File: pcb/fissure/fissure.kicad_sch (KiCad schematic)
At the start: 64 parts, among them J1 Conn_01x04_Female, J2 USB_C_Receptacle_USB2.0, J3 Conn_01x06, J4 Conn_01x06, J5 OLED, J6 Conn_01x06, J7 Conn_01x06, K1 KEY, K10 KEY, K11 KEY, K12 KEY, K13 KEY, K14 KEY, K15 KEY, K16 KEY, K17 KEY, K18 KEY, K19 KEY, K2 KEY, K20 KEY, K3 KEY, K4 KEY, K5 KEY, K6 KEY, K7 KEY, K8 KEY, K9 KEY, Q1 AO3401A, Q2 AO3401A, SW1 SW_Push, SW2 SW_Push, SW3 SW_SPDT, SW4 SW_SPDT, U1 Holyiot_18010, U2 MT25QL128ABA1ESE, U3 LTC4054ES5-4.2, U4 MCP1700-3302E_SOT23

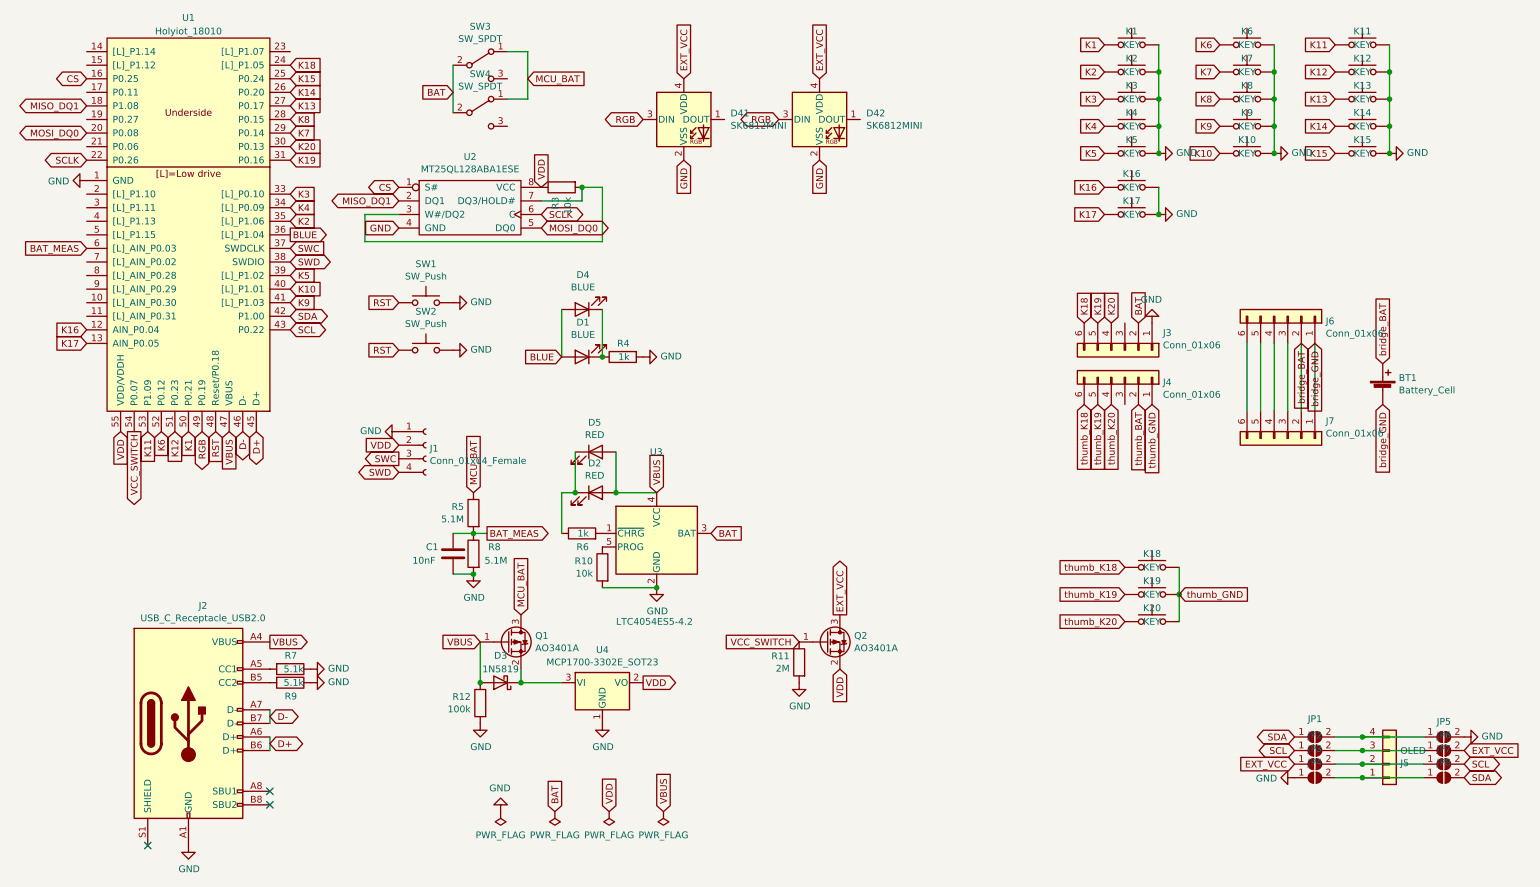
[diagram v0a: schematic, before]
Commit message: Backup
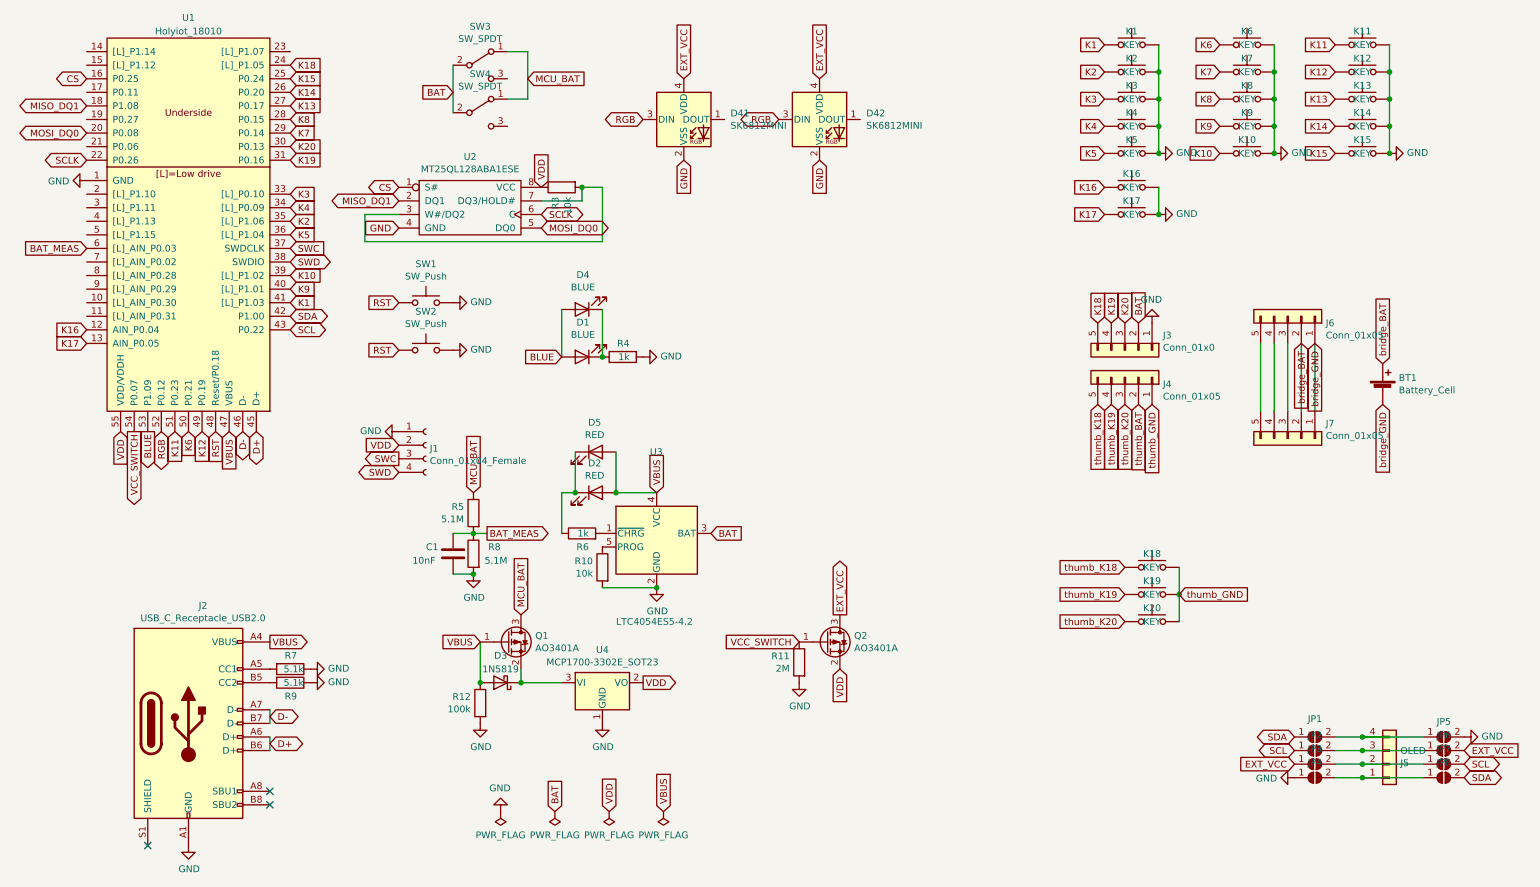
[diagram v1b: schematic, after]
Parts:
- removed J3, J4: Conn_01x06, fissure:bridge-conn, symbol Connector_Generic:Conn_01x06
- removed J6, J7: Conn_01x06, fissure:bridge, symbol Connector_Generic:Conn_01x06
- added J3: Conn_01x0, fissure:bridge-conn, symbol Connector_Generic:Conn_01x05
- added J4: Conn_01x05, fissure:bridge-conn, symbol Connector_Generic:Conn_01x05
- added J6, J7: Conn_01x05, fissure:bridge, symbol Connector_Generic:Conn_01x05
- D1, D2, D4, D5: footprint LED_SMD:LED_1206_3216Metric -> LED_SMD:LED_0805_2012Metric
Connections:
- net BAT: now also J3.2 (Pin_2)
- net BLUE: now also U1.53 (P1.09); no longer U1.36 ([L]_P1.04)
- net GND: now also J3.1 (Pin_1)
- net K1: now also U1.41 ([L]_P1.03); no longer U1.50 (P0.21)
- net K10: now also U1.39 ([L]_P1.02); no longer U1.40 ([L]_P1.01)
- net K11: now also U1.51 (P0.23); no longer U1.53 (P1.09)
- net K12: now also U1.49 (P0.19); no longer U1.51 (P0.23)
- net K18: now also J3.5 (Pin_5)
- net K19: now also J3.4 (Pin_4)
- net K20: now also J3.3 (Pin_3)
- net K5: now also U1.36 ([L]_P1.04); no longer U1.39 ([L]_P1.02)
- net K6: now also U1.50 (P0.21); no longer U1.52 (P0.12)
- net K9: now also U1.40 ([L]_P1.01); no longer U1.41 ([L]_P1.03)
- net RGB: now also U1.52 (P0.12); no longer U1.49 (P0.19)
- net bridge_BAT: now also J6.2 (Pin_2), J7.2 (Pin_2)
- net bridge_GND: now also J6.1 (Pin_1), J7.1 (Pin_1)
- net thumb_BAT: now also J4.2 (Pin_2)
- net thumb_GND: now also J4.1 (Pin_1)
- net thumb_K18: now also J4.5 (Pin_5)
- net thumb_K19: now also J4.4 (Pin_4)
- net thumb_K20: now also J4.3 (Pin_3)
- new net: J6.3 (Pin_3), J7.3 (Pin_3)
- new net: J6.4 (Pin_4), J7.4 (Pin_4)
- new net: J6.5 (Pin_5), J7.5 (Pin_5)
